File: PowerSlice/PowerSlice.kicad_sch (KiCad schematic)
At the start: 32 parts, among them J1 Conn_01x10_Pin, J2 DC_In_Barrel, J3 DC_In_Screw, J4 ESTOP, U1 PTH08080WAD, U2 PTH08080WAD, U3 INA214BIDCKR, U4 INA214BIDCKR, U5 INA214BIDCKR, U6 NUCLEO-F303K8

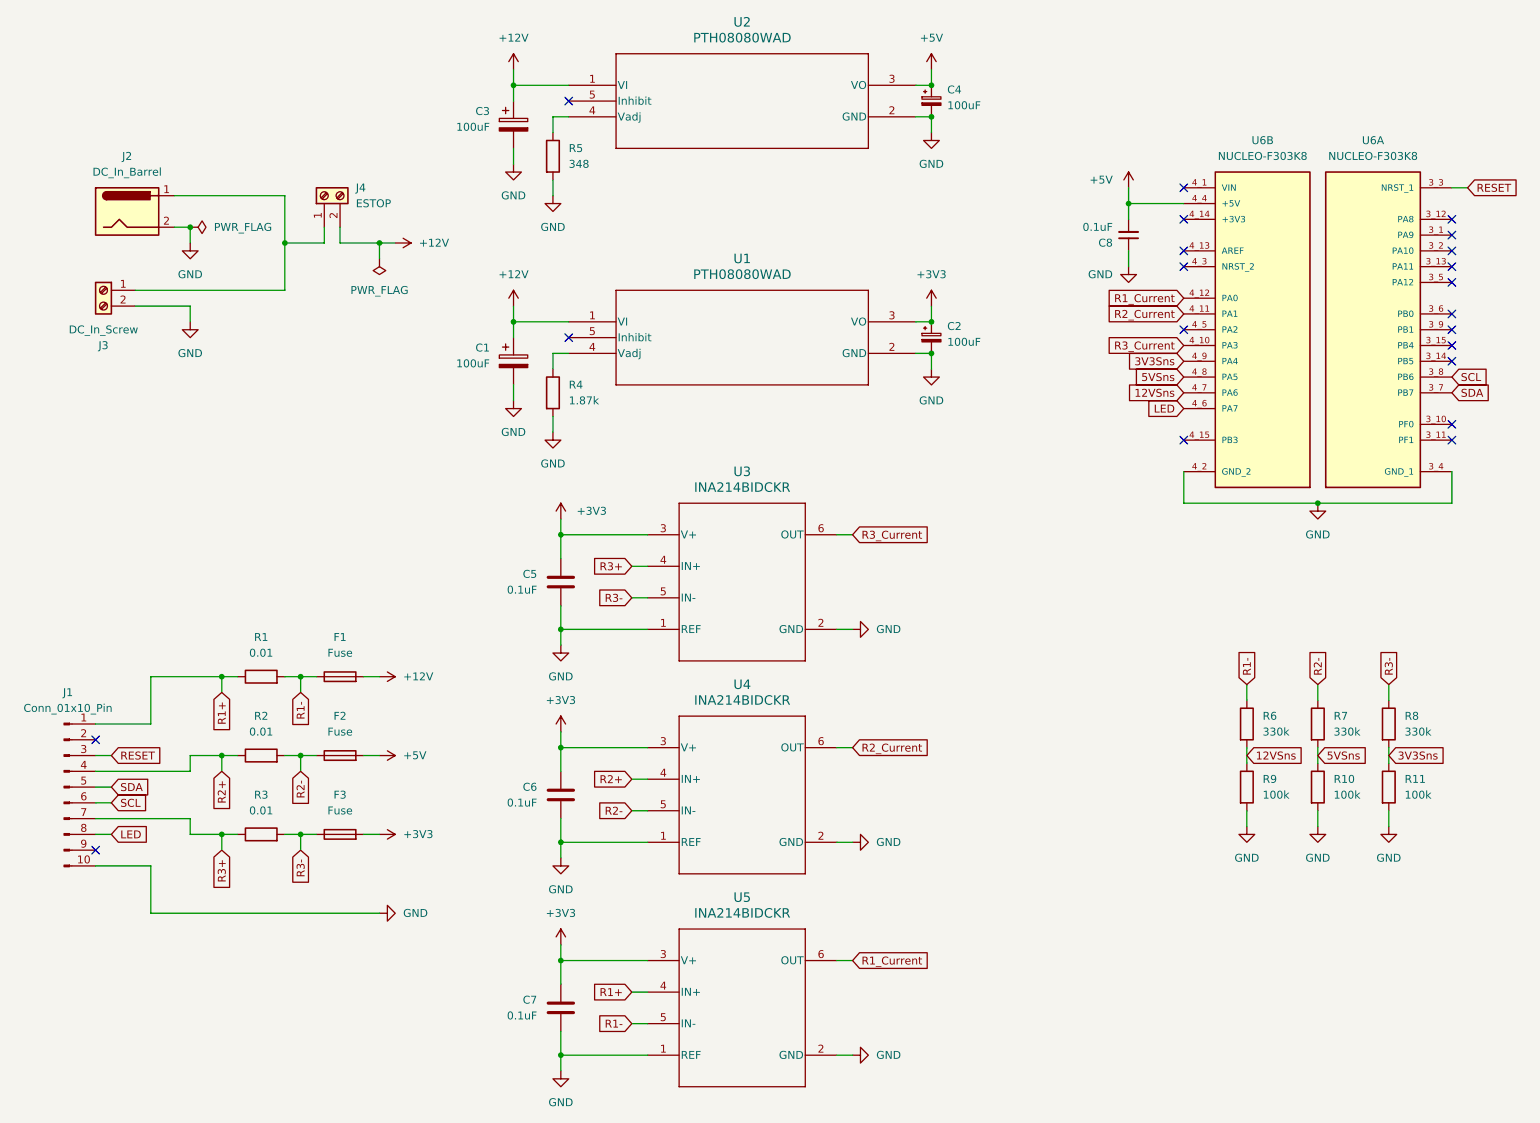
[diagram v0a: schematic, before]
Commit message: Wacky stuff that needs to be changed cuz it wont work and will be reverted
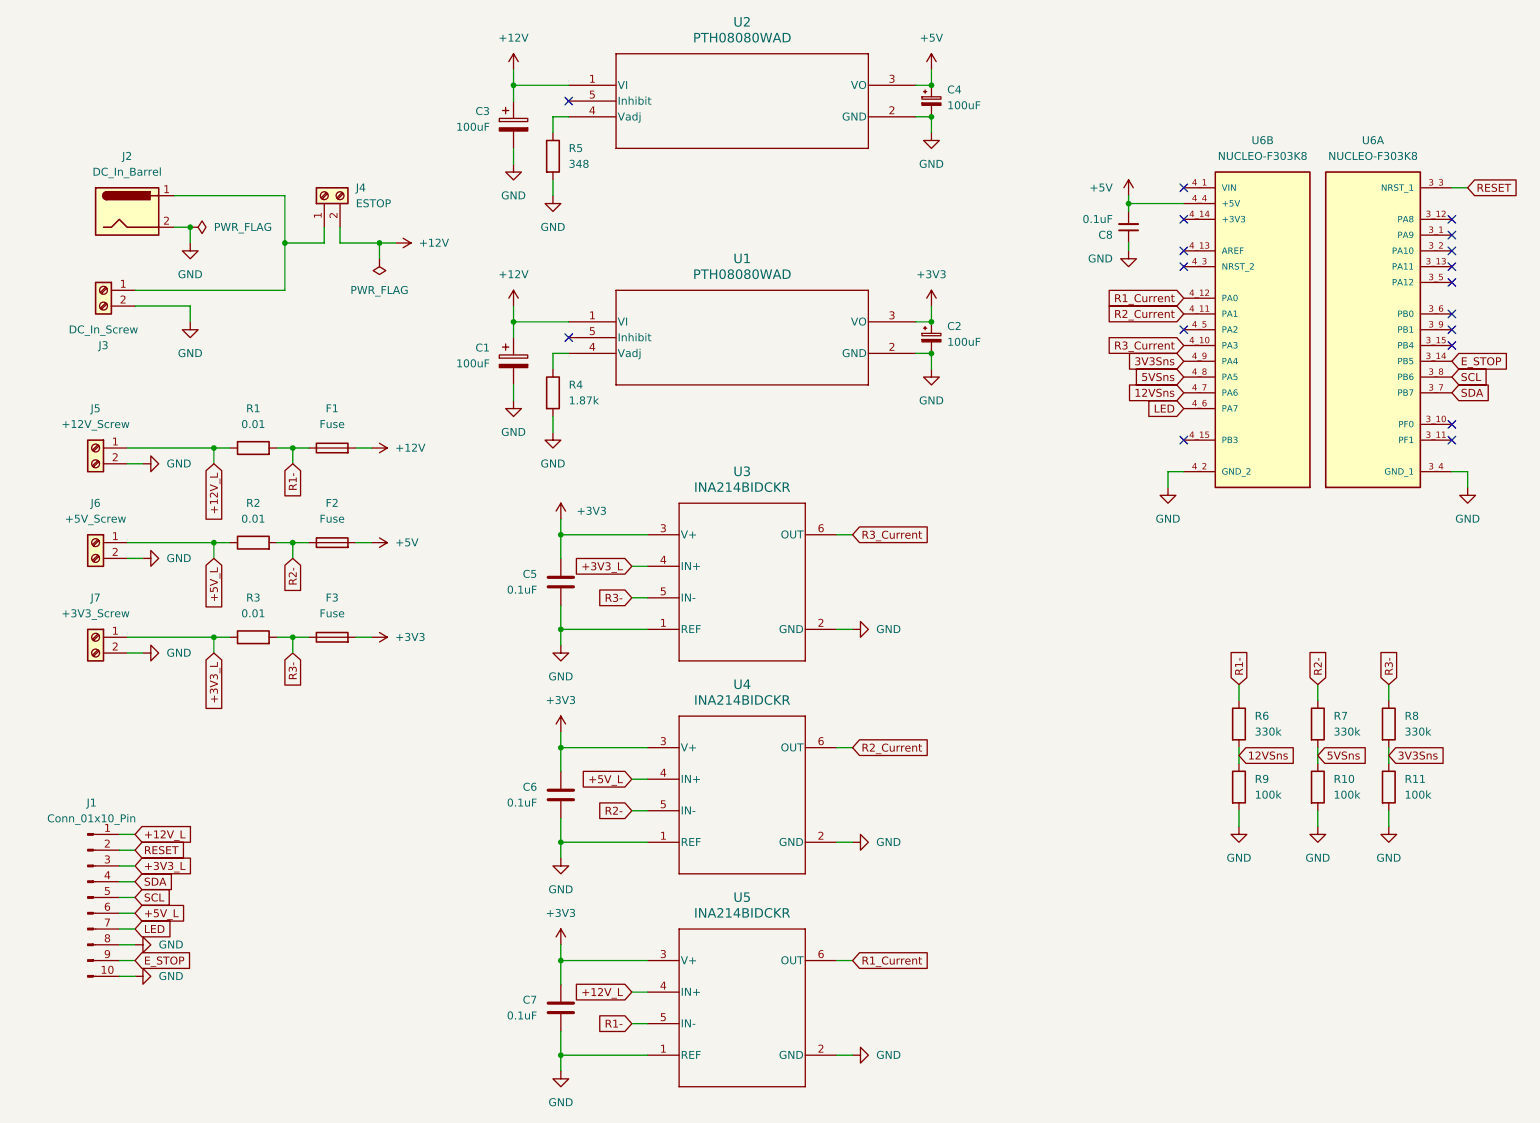
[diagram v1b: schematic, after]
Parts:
- added J5: +12V_Screw, 691137710002:691137710002, symbol Connector:Screw_Terminal_01x02
- added J6: +5V_Screw, 691137710002:691137710002, symbol Connector:Screw_Terminal_01x02
- added J7: +3V3_Screw, 691137710002:691137710002, symbol Connector:Screw_Terminal_01x02
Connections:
- net GND: now also J1.8 (Pin_8), J5.2 (Pin_2), J6.2 (Pin_2), J7.2 (Pin_2)
- net LED: now also J1.7 (Pin_7); no longer J1.8 (Pin_8)
- net RESET: now also J1.2 (Pin_2); no longer J1.3 (Pin_3)
- net SCL: now also J1.5 (Pin_5); no longer J1.6 (Pin_6)
- net SDA: now also J1.4 (Pin_4); no longer J1.5 (Pin_5)
- net E_STOP: now reaches J1.9 (Pin_9)
- net E_STOP: now also U6.3_14 (PB5)
- net R1+ renamed +12V_L
- net +12V_L: now also J5.1 (Pin_1)
- net R2+ renamed +5V_L
- net +5V_L: now also J1.6 (Pin_6), J6.1 (Pin_1); no longer J1.4 (Pin_4)
- net R3+ renamed +3V3_L
- net +3V3_L: now also J1.3 (Pin_3), J7.1 (Pin_1); no longer J1.7 (Pin_7)
- no-connect marks 21 -> 18
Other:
- moved on the sheet: C8, F1, F2, F3, J1, R1, R2, R3, R6, R9

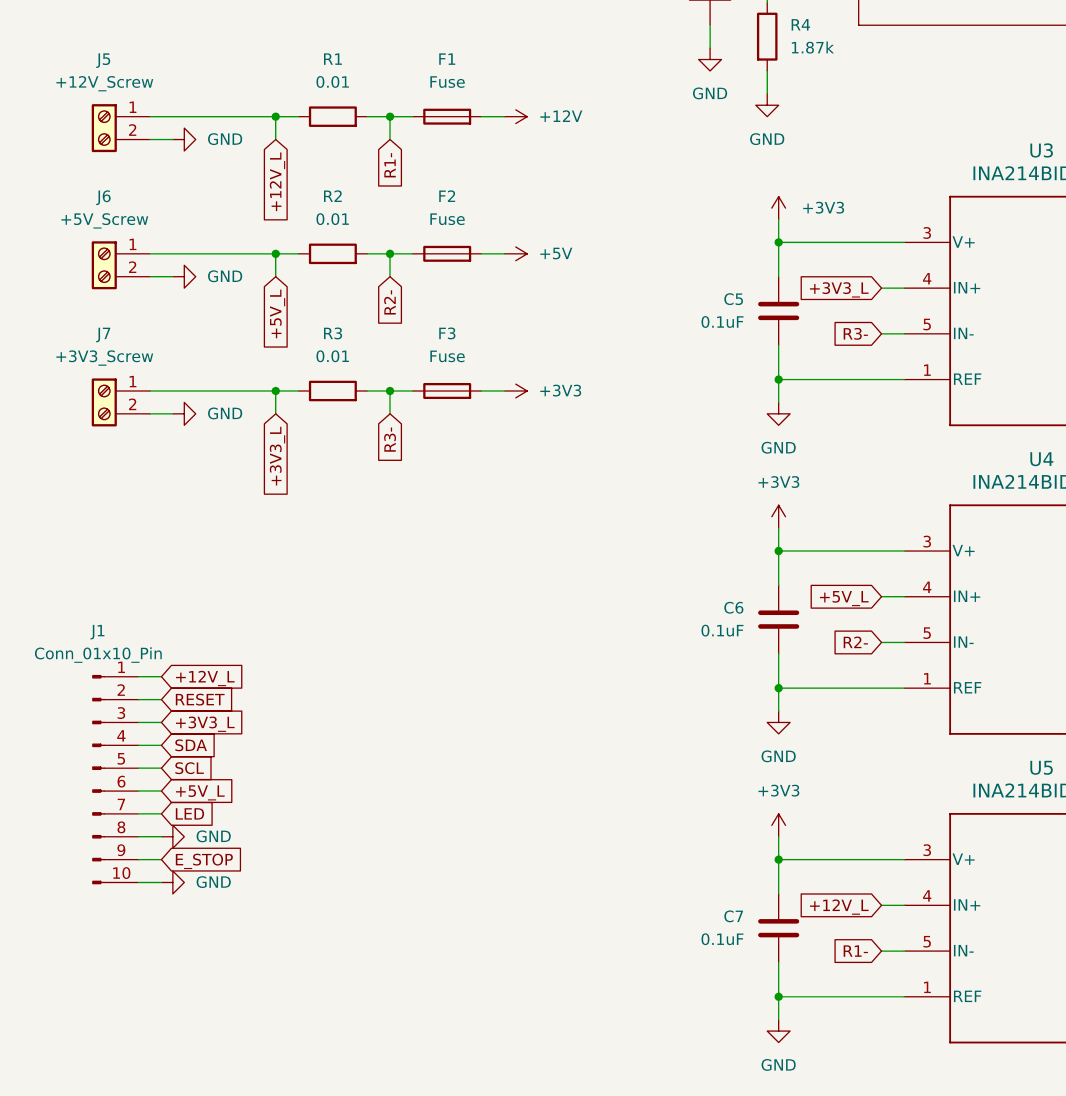
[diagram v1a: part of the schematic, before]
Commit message: Work, TODO: figure out external power connectors
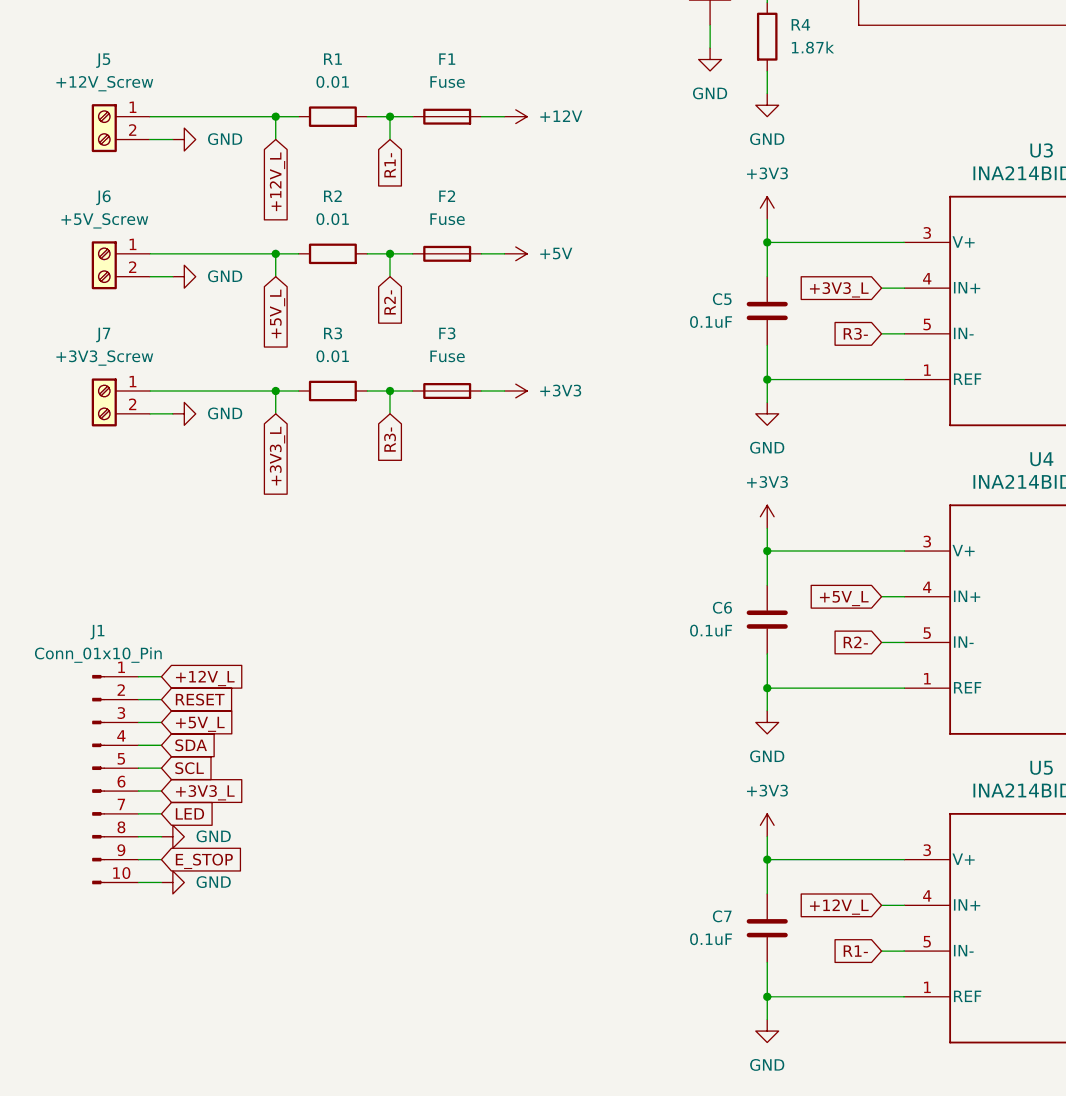
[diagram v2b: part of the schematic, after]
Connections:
- net +3V3_L: now also J1.6 (Pin_6); no longer J1.3 (Pin_3)
- net +5V_L: now also J1.3 (Pin_3); no longer J1.6 (Pin_6)
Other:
- moved on the sheet: C5, C6, C7
